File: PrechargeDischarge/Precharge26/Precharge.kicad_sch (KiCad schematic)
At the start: 119 parts, among them J1 MicroFit, J2 Mini-Fit_Jr_5566-04A, J3 Micro-Fit 43045-0212, J4 Micro-Fit 43045-0212, K1 OMRON-G2RL-24, K2 G7L-2A-X-L, K4 Relay_SPST-NC, Q1 2N7002, Q2 MMBT3906, Q3 2N7002, Q5 NMOS, U1 TJA1051T-3, U10 LM393, U11 4N35, U2 SPAN02A-12, U3 Teensy4.0, U4 LM1117-5.0, U5 4N35, U6 4N35, U7 LM331, U8 LM331, U9 LM2904

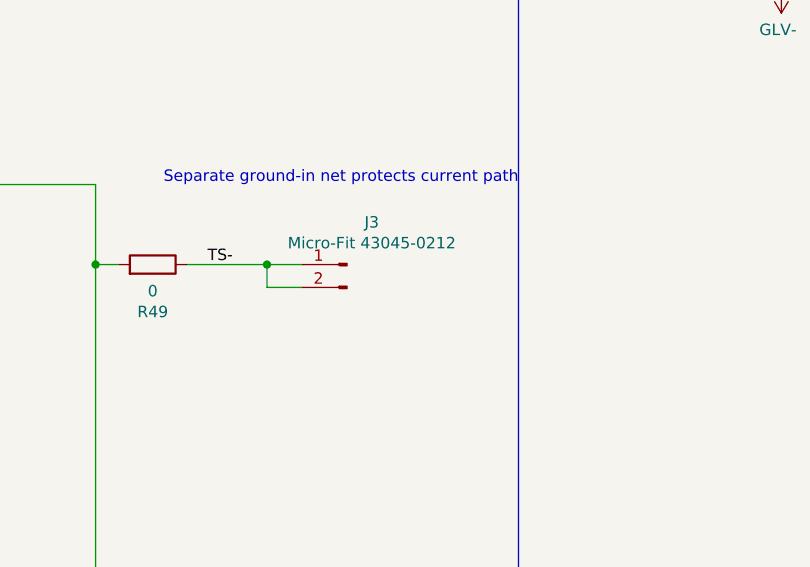
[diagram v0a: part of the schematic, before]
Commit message: Molex Microfit
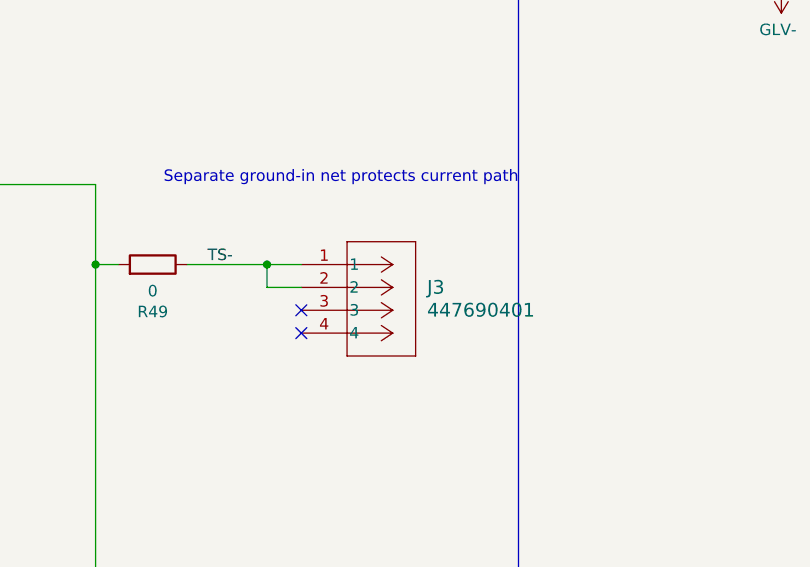
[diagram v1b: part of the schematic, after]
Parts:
- removed J3: Micro-Fit 43045-0212, Connector_Molex:Molex_Micro-Fit_3.0_43045-0212_2x01_P3.00mm_Vertical, symbol Connector:Conn_01x02_Pin
- added J3: 447690401, Precharge:MICROFIT-4PIN, symbol precharge-lib 2:447690401
- J2: footprint Mini-Fit-Jr-4.20mm-pitch:Molex-Mini-Fit-Jr-4-pin-P4.2mm-RowP4.2mm -> Precharge:MICROFIT-4PIN
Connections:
- net TS-: now also J3.1, J3.2
- no-connect marks 12 -> 14
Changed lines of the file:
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@@
 	)
 	(no_connect
+		(at 270.51 322.58)
+	)
+	(no_connect
 		(at 36.83 229.87)
 	)
@@
 	)
 	(no_connect
+		(at 270.51 325.12)
+	)
+	(no_connect
 		(at 27.94 162.56)
 	)
@@
 			"AGMAKwBkAE8AbgB6ADYAZABrADUAUAB6AHcAUQBjAGYATABGADIANgA5AEsATwBQAFAAdABxAHkA"
 			"WgBZAHYAUAA1ADQAUABvAGkATQBsAFMAYgBSADgAZgBSACsATQBDAEoANAA0AGMASABCAHcAMQBE"
-			"AGoAQQBWAHAAVgBLAEoAVQBEAFgAVgBvADEAUQBYAHcASABXAGcAYQBQAHIAOQ=="
+			"AGoAQQBWAHAAVgBLAEoAVQBEAFgAVgBvADEAUQBYAHcASABXAGcAYQBQAHIAOf/Qxaz/0MWs/9DF"
+			"rP/Qxaz/0MWs/9DFrP/Qxaz/0MWs/9DFrP/Qxaz/0MWs/9DFrP/Qxaz/0MWs/9DFrP/Qxaz/0MWs"
+			"/9DFrP/Qxaz/0MWs/9DFrP/Qxaz/0MWs/9DFrP/Qxaz/0MWs/9DFrP/Qxaz/0MWs/9DFrP/Qxaz/"
+			"0MWs/9DFrP/Qxaz/0MWs/9DFrP/Qxaz/0MWs/9DFrP/Qxaz/0MWs/9DFrP/Qxaz/0MWs/9DFrP/Q"
+			"xaz/0MWs/9DFrP/Qxaz/0MWs/9DFrP/Qxaz/0MWs/9DFrP/Qxaz/0MWs/9DFrP9+enL/VFRU/1RU"
+			"VP9UVFT/VFRU/1RUVP9UVFT/VFRU/1RUVP9UVFT/VFRU/9DFrP/Qxaz/0MWs/9DFrP/Qxaz/0MWs"
+			"/9DFrP/Qxaz/0MWs/9DFrP/Qxaz/0MWs/9DFrP/Qxaz/0MWs/9DFrP/Qxaz/0MWs/9DFrP/Qxaz/"
+			"0MWs/9DFrP/Qxaz/0MWs/9DFrP/Qxaz/0MWs/9DFrP/Qxaz/0MWs/9DFrP/Qxaz/0MWs/9DFrP/Q"
+			"xaz/0MWs/9DFrP/Qxaz/0MWs/9DFrP/Qxaz/0MWs/9DFrP/Qxaz/0MWs/9DFrP/Qxaz/0MWs/9DF"
+			"rP/Qxaz/0MWs/9DFrP/Qxaz/0MWs/9DFrP/Qxaz/0MWs/9DFrP/Qxaz/0MWs/9DFrP/Qxaz/0MWs"
+			"/9DFrP/Qxaz/0MWs/9DFrP/Qxaz/0MWs/9DFrP/Qxaz/0MWs/9DFrP/Qxaz/0MWs/9DFrP/Qxaz/"
+			"0MWs/9DFrP/Qxaz/0MWs/9DFrP/Qxaz/0MWs/9DFrP/Qxaz/0MWs/9DFrP/Qxaz/0MWs/9DFrP/Q"
+			"xaz/0MWs/9DFrP/Qxaz/0MWs/9DFrP/Qxaz/0MWs/9DFrP/Qxaz/0MWs/9DFrP/Qxaz/0MWs/9DF"
+			"rP/Qxaz/0MWs/9DFrP/Qxaz/0MWs/9DFrP/Qxaz/0MWs/9DFrP/Qxaz/0MWs/9DFrP/Qxaz/0MKq"
+			"NgAAAAAAAAAAAAAAAAAAAAAAAAAAAAAAAAAAAAAAAAAAAAAAAAAAAAAAAAAAAAAAAAAAAAAAAAAA"
+			"AAAAAAAAAAAAAAAAz8SrhdDFrP/Qxaz/0MWs/9DFrP/Qxaz/0MWs/9DFrP/Qxaz/0MWs/9DFrP/Q"
+			"xaz/0MWs/9DFrP/Qxaz/0MWs/9DFrP/Qxaz/0MWs/9DFrP/Qxaz/0MWs/9DFrP/Qxaz/0MWs/9DF"
+			"rP/Qxaz/0MWs/9DFrP/Qxaz/0MWs/9DFrP/Qxaz/0MWs/9DFrP/Qxaz/0MWs/9DFrP/Qxaz/0MWs"
+			"/9DFrP/Qxaz/0MWs/9DFrP/Qxaz/0MWs/9DFrP/Qxaz/0MWs/9DFrP/Qxaz/0A=="
 		)
 	)
@@
 	)
 	(symbol
-		(lib_id "Connector:Conn_01x02_Pin")
-		(at 275.59 317.5 0)
-		(mirror y)
-		(unit 1)
-		(exclude_from_sim no)
-		(in_bom yes)
-		(on_board yes)
-		(dnp no)
-		(property "Reference" "J3"
-			(at 278.3332 312.801 0)
-			(effects
-				(font
-					(size 1.27 1.27)
-				)
-			)
-		)
-		(property "Value" "Micro-Fit 43045-0212"
-			(at 278.3332 315.1124 0)
-			(effects
-				(font
-					(size 1.27 1.27)
-				)
-			)
-		)
-		(property "Footprint" "Connector_Molex:Molex_Micro-Fit_3.0_43045-0212_2x01_P3.00mm_Vertical"
-			(at 275.59 317.5 0)
-			(effects
-				(font
-					(size 1.27 1.27)
-				)
-				(hide yes)
-			)
-		)
-		(property "Datasheet" "~"
-			(at 275.59 317.5 0)
-			(effects
-				(font
-					(size 1.27 1.27)
-				)
-				(hide yes)
-			)
-		)
-		(property "Description" "Generic connector, single row, 01x02, script generated"
-			(at 275.59 317.5 0)
-			(effects
-				(font
-					(size 1.27 1.27)
-				)
-				(hide yes)
-			)
-		)
-		(property "JLC" ""
-			(at 275.59 317.5 0)
-			(effects
-				(font
-					(size 1.27 1.27)
-				)
-				(hide yes)
-			)
-		)
-		(property "MFR" ""
-			(at 275.59 317.5 0)
-			(effects
-				(font
-					(size 1.27 1.27)
-				)
-				(hide yes)
-			)
-		)
-		(pin "1"
-		)
-		(pin "2"
-		)
-		(instances
-			(project ""
-				(path "/56395b7f-8d0b-4695-8aad-21fefa44f8f8"
-					(reference "J3")
-					(unit 1)
-				)
-			)
-		)
-	)
-	(symbol
 		(lib_id "Isolator:4N35")
 		(at 55.88 300.99 0)
@@
 			)
 		)
-		(property "Footprint" "Mini-Fit-Jr-4.20mm-pitch:Molex-Mini-Fit-Jr-4-pin-P4.2mm-RowP4.2mm"
+		(property "Footprint" "Precharge:MICROFIT-4PIN"
 			(at 31.75 229.87 0)
 			(effects
@@
 					(unit 1)
 				)
+			)
+		)
+	)
+	(symbol
+		(lib_id "precharge-lib 2:447690401")
+		(at 270.51 317.5 0)
+		(unit 1)
+		(exclude_from_sim no)
+		(in_bom yes)
+		(on_board yes)
+		(dnp no)
+		(fields_autoplaced yes)
+		(property "Reference" "J3"
+			(at 284.48 320.0399 0)
+			(effects
+				(font
+					(size 1.524 1.524)
+				)
+				(justify left)
+			)
+		)
+		(property "Value" "447690401"
+			(at 284.48 322.5799 0)
+			(effects
+				(font
+					(size 1.524 1.524)
+				)
+				(justify left)
+			)
+		)
+		(property "Footprint" "Precharge:MICROFIT-4PIN"
+			(at 270.51 317.5 0)
+			(effects
+				(font
+					(size 1.27 1.27)
+					(italic yes)
+				)
+				(hide yes)
+			)
+		)
+		(property "Datasheet" "https://www.molex.com/en-us/products/part-detail-pdf/447690401?display=pdf"
+			(at 270.51 317.5 0)
+			(effects
+				(font
+					(size 1.27 1.27)
+					(italic yes)
+				)
+				(hide yes)
+			)
+		)
+		(property "Description" ""
+			(at 270.51 317.5 0)
+			(effects
+				(font
+					(size 1.27 1.27)
+				)
+				(hide yes)
+			)
+		)
+		(pin "4"
+		)
+		(pin "3"
+		)
+		(pin "1"
+		)
+		(pin "2"
+		)
+		(instances
+			(project ""
+				(path "/56395b7f-8d0b-4695-8aad-21fefa44f8f8"
+					(reference "J3")
+					(unit 1)
+				)
